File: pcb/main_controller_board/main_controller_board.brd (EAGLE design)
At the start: 72.1 x 52.1 mm, 50 parts, among them K1 61400416021, U1 RPI_CAMERA, U2 RPI_CAMERA

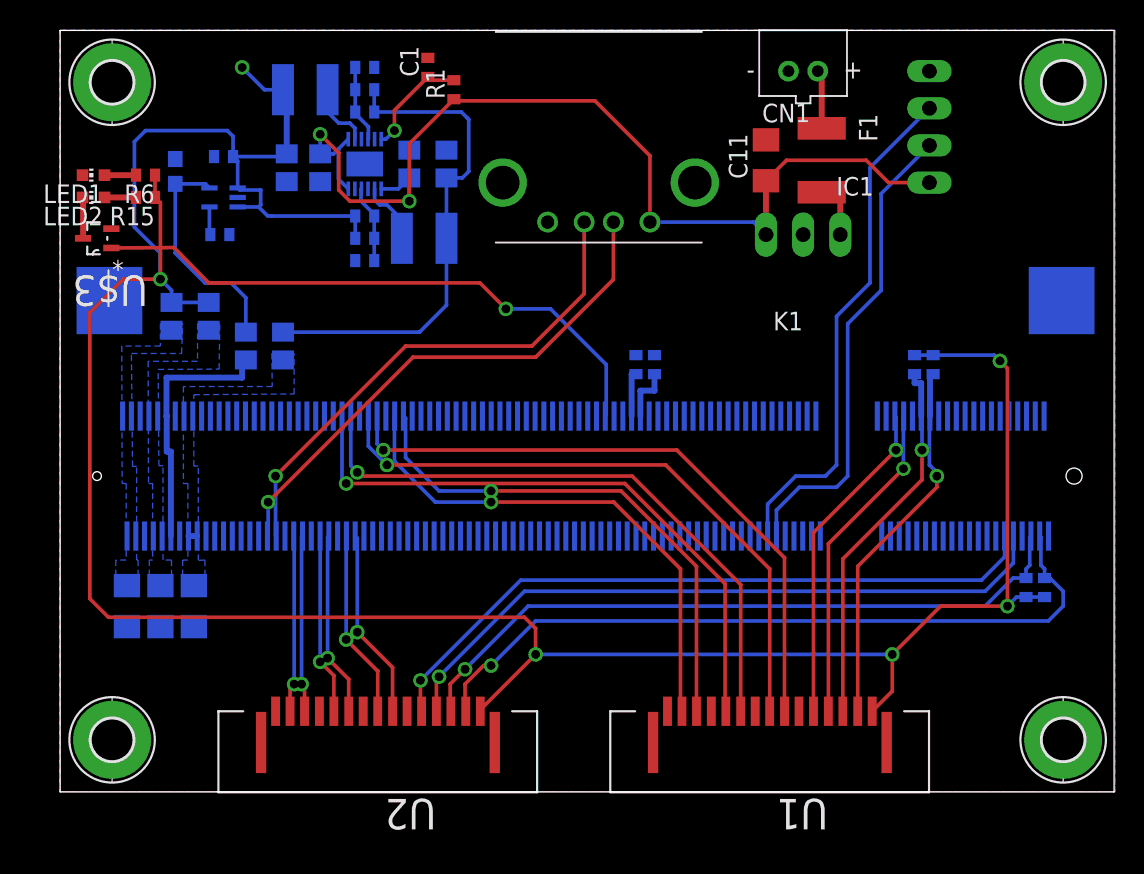
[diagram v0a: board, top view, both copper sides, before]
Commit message: rev0.1
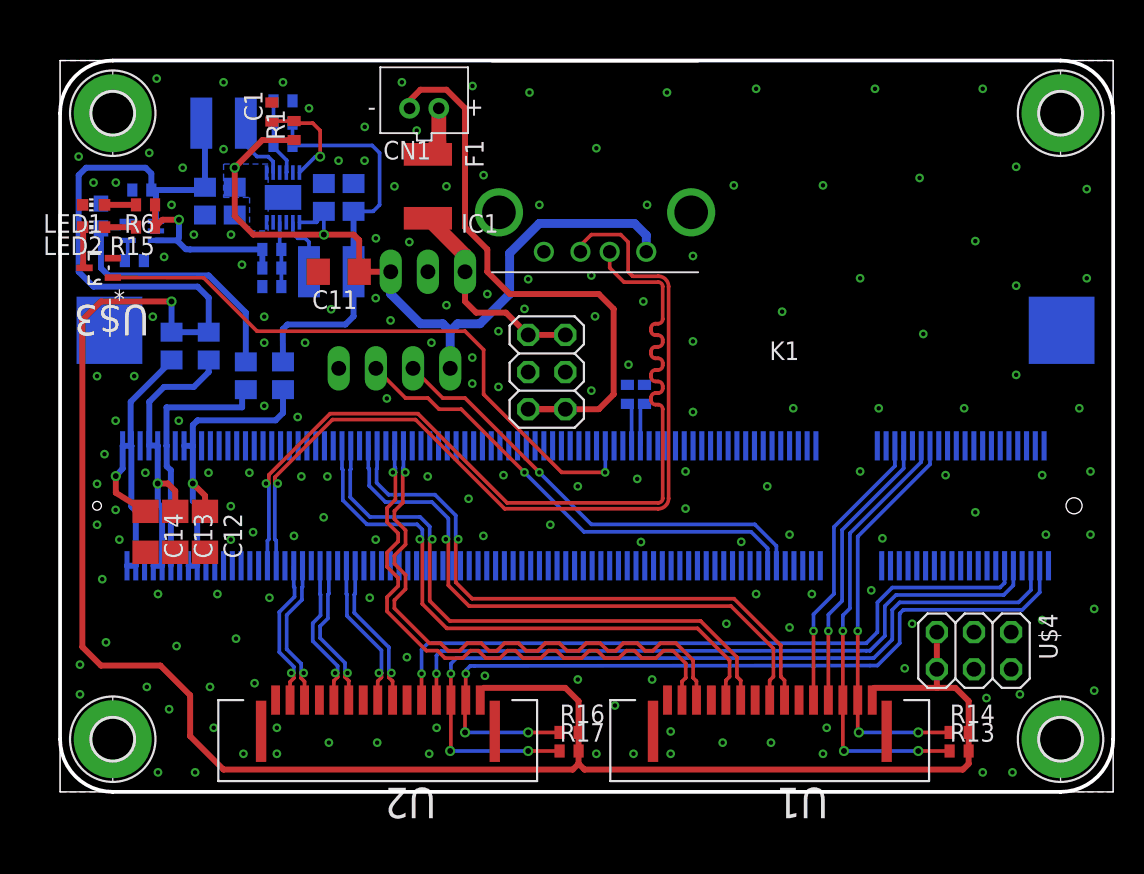
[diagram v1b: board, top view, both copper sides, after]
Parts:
- added U$4: TENDA_P200, openblw:TENDA_P200
- moved JP1 40.1 mm to (22.9, 29.0), turned to 0 degrees
- moved R16 34.0 mm to (34.8, 4.06), flipped to the top, turned to 0 degrees
- moved R17 33.2 mm to (34.8, 2.79), flipped to the top, turned to 0 degrees
- moved C11 30.2 mm to (19.1, 35.6), turned to 180 degrees
- moved F1 27.0 mm to (25.1, 41.4)
- moved R13 26.6 mm to (61.5, 2.79), flipped to the top, turned to 0 degrees
- moved CN1 26.0 mm to (24.9, 46.7)
- moved IC1 25.8 mm to (25.1, 33.0)
- moved R14 25.2 mm to (61.5, 4.06), flipped to the top, turned to 0 degrees
- moved R1 11.3 mm to (16.0, 45.2)
- moved C1 11.1 mm to (14.5, 46.5)
- moved C7 6.75 mm to (20.1, 40.6)
- moved R2 6.75 mm to (14.5, 37.1)
- moved L2 6.75 mm to (18.5, 35.6)
- moved C4 6.67 mm to (14.5, 35.8)
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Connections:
- net CAM0_CN renamed CAM0_C_N
- net CAM0_CP renamed CAM0_C_P
- net CAM0_DN0 renamed CAM0_D0_N
- net CAM0_DN1 renamed CAM0_D1_N
- net CAM0_DP0 renamed CAM0_D0_P
- net CAM0_DP1 renamed CAM0_D1_P
- net CAM1_CN renamed CAM1_C_N
- net CAM1_CP renamed CAM1_C_P
- net CAM1_DN0 renamed CAM1_D0_N
- net CAM1_DN1 renamed CAM1_D1_N
- net CAM1_DP0 renamed CAM1_D0_P
- net CAM1_DP1 renamed CAM1_D1_P
- net USB_DN renamed USB_D_N
- net USB_DP renamed USB_D_P
- new net DGND: U$4.5, U$4.6
- net +12V: now also U$4.1, U$4.2
- net +3V3: now also U$4.7, U$4.8
- net GND: now also U$4.12
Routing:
- net DGND: track 0.00 -> 41.3 mm
- net USB_D_P: track 35.3 -> 61.8 mm
- net USB_D_N: track 36.2 -> 61.1 mm
- net CM_VBAT: track 0.00 -> 22.4 mm, vias 0 -> 1
- net CM_3V3: track 0.48 -> 21.2 mm, vias 0 -> 1
- net CM_1V8: track 0.83 -> 21.3 mm, vias 0 -> 1
- net +5V: track 72.1 -> 55.4 mm
- net CAM1_SCL: track 47.3 -> 58.5 mm, vias 1 -> 3
- net +12V: track 4.16 -> 14.5 mm
- net +3V3: track 185.0 -> 178.7 mm, vias 6 -> 2
- net +1V8: track 34.1 -> 28.6 mm
- net CAM0_D0_N: track 35.5 -> 40.2 mm
- net CAM1_SDA: track 50.6 -> 55.2 mm, vias 1 -> 3
- net CAM0_SCL: track 25.8 -> 30.3 mm, vias 1 -> 3
- net CAM0_D0_P: track 35.8 -> 40.2 mm
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- added copper zone on layer 16, net +5V
- removed copper zone on layer 16, net CM_1V8
- removed copper zone on layer 16, net CM_3V3
- removed copper zone on layer 16, net CM_VBAT
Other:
- board size 72.1 x 52.1 mm -> 72 x 50 mm
